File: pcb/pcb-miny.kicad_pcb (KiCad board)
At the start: 2 copper layers, 139.8 x 99.8 mm, 116 parts, among them SW1 Switch, SW10 Switch, SW11 Switch, SW12 Switch, SW13 Switch, SW14 Switch, SW15 Switch, SW16 Switch, SW17 Switch, SW18 Switch, SW19 Switch, SW2 Switch, SW20 Switch, SW21 Switch, SW22 Switch, SW23 Switch, SW24 Switch, SW25 Switch, SW26 Switch, SW27 Switch, SW28 Switch, SW29 Switch, SW3 Switch, SW30 Switch, SW31 Switch, SW32 Switch, SW33 Switch, SW34 Switch, SW4 Switch, SW5 Switch, SW6 Switch, SW7 Switch, SW8 Switch, SW9 Switch

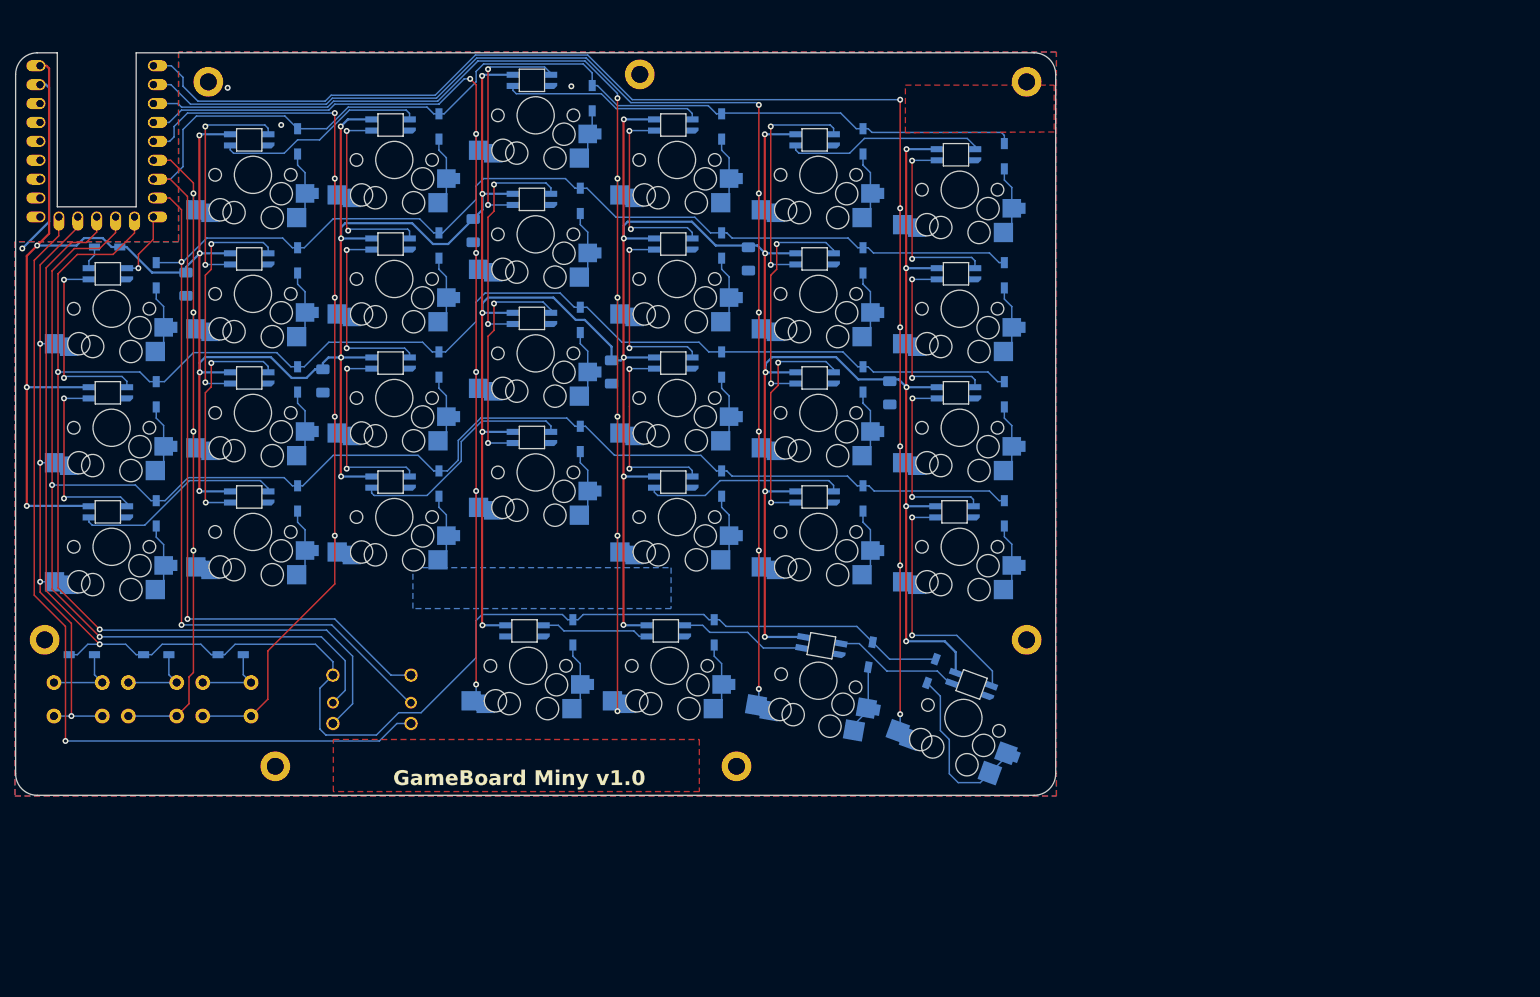
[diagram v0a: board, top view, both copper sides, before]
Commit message: miny-v2 draft
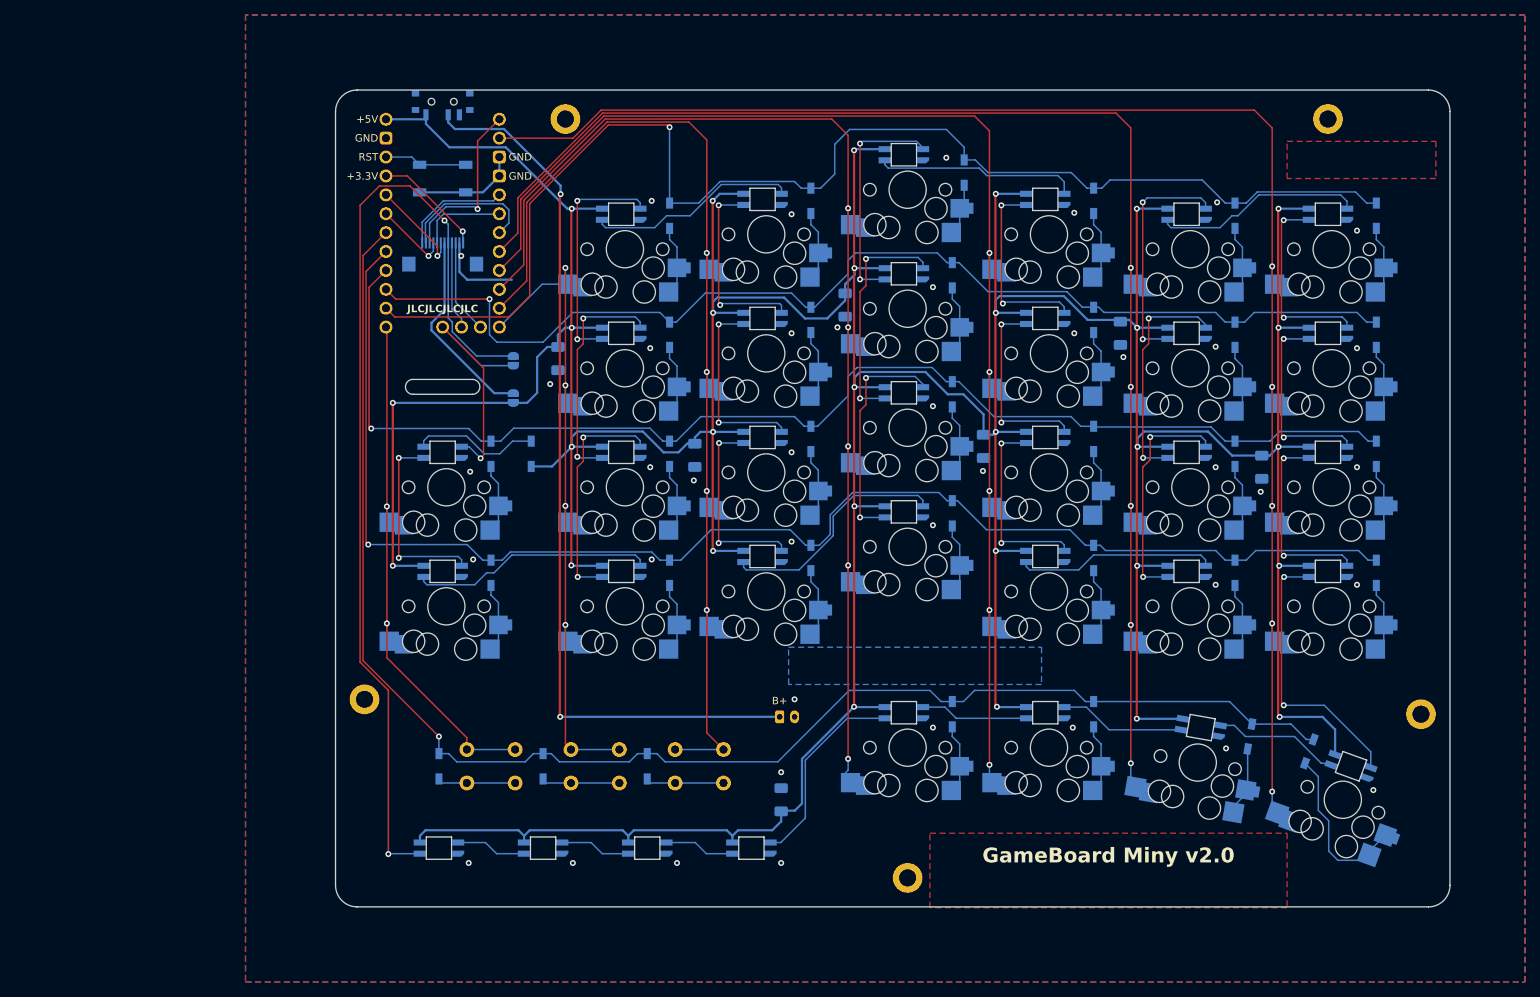
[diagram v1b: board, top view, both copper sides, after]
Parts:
- removed the D7 at (36.5, 100.5)
- removed FiveWay1: 5Way-Tactile_K1-1506DN-01, zzkeeb:Button_5way
- removed the H4 at (101.5, 73.5)
- removed H6: MountingHole, zzkeeb:Hole_M2-TH
- removed the LED1 at (30.0, 100.3)
- removed MCU1: rp2040-zero, zzkeeb:MCU_rp2040-zero-tht
- removed the SW7 at (30.5, 105.0)
- added C7: 100n, Capacitor_SMD:C_1206_3216Metric_Pad1.33x1.80mm_HandSolder, B.Cu at (120.5, 171.0)
- added J1: RP2040, zzkeeb:MCU_rp2040-helios, B.Cu at (75.0, 93.5)
- added J2: Conn_01x02_Socket, zzkeeb:Connector_JST-1x02-2.00mm, F.Cu at (120.3, 159.8)
- added JP2: VIK 5V, Jumper:SolderJumper-2_P1.3mm_Open_RoundedPad1.0x1.5mm, B.Cu at (84.5, 117.0)
- added JP4: VIK LED, Jumper:SolderJumper-2_P1.3mm_Open_RoundedPad1.0x1.5mm, B.Cu at (84.5, 112.0)
- added LED31: YS-SK6812MINI-E, zzkeeb:LED_SK6812-MINI-E, B.Cu at (116.5, 177.5)
- added LED32: YS-SK6812MINI-E, zzkeeb:LED_SK6812-MINI-E, B.Cu at (102.5, 177.5)
- added LED33: YS-SK6812MINI-E, zzkeeb:LED_SK6812-MINI-E, B.Cu at (88.5, 177.5)
- added LED34: YS-SK6812MINI-E, zzkeeb:LED_SK6812-MINI-E, B.Cu at (74.5, 177.5)
- added RST1: SW_Push, zzkeeb:Button_SW_SPST_SKQG_WithoutStem, B.Cu at (75.0, 87.5)
- added SW34: SW_SPDT, zzkeeb:Switch_SPDT-PCM12, B.Cu at (75.0, 77.5)
- added VIK_K1: Connector_VIK-keyboard, zzkeeb:Connector_VIK-horizontal-keyboard, B.Cu at (75.0, 97.7)
- moved SW29 64.1 mm to (109.5, 166.5), turned to 180 degrees
- moved D34 63.4 mm to (86.9, 124.5), turned to -90 degrees
- moved SW28 60.2 mm to (95.5, 166.5), turned to 180 degrees
- moved D29 58.0 mm to (102.5, 166.5), turned to -90 degrees
- moved SW27 56.2 mm to (81.5, 166.5), turned to 180 degrees
- moved D28 54.1 mm to (88.5, 166.5), turned to -90 degrees
- moved H5 53.9 mm to (206.5, 159.5)
- moved D30 52.2 mm to (143.5, 159.5)
- moved D31 52.2 mm to (162.5, 159.5)
- moved D32 52.2 mm to (183.5, 162.5)
- moved LED27 52.2 mm to (197.1, 166.5)
- moved LED28 52.2 mm to (176.9, 161.3)
- moved LED29 52.2 mm to (156.0, 159.3)
- moved LED30 52.2 mm to (137.0, 159.3)
- moved SW30 52.2 mm to (137.5, 164.0)
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- renumbered D11 to D10, D12 to D11, D13 to D12, D14 to D13, D15 to D14, D16 to D15, D17 to D16, D18 to D17, D19 to D18, D20 to D19, D21 to D20, D22 to D21, D23 to D22, D24 to D23, D25 to D24, D26 to D25, D27 to D26, D28 to D27, D29 to D28, D30 to D29, D31 to D30, D32 to D31, D33 to D32, D34 to D33, D40 to D34, D8 to D7, D9 to D8, D10 to D9, H7 to H4, LED2 to LED1, LED11 to LED10, LED12 to LED11, LED13 to LED12, LED14 to LED13, LED15 to LED14, LED16 to LED15, LED17 to LED16, LED18 to LED17, LED19 to LED18, LED20 to LED19, LED3 to LED2, LED21 to LED20, LED22 to LED21, LED23 to LED22, LED24 to LED23, LED25 to LED24, LED26 to LED25, LED27 to LED26, LED28 to LED27, LED29 to LED28, LED30 to LED29, LED4 to LED3, LED31 to LED30, LED5 to LED4, LED6 to LED5, LED7 to LED6, LED8 to LED7, LED9 to LED8, LED10 to LED9, SW11 to SW10, SW12 to SW11, SW13 to SW12, SW14 to SW13, SW15 to SW14, SW16 to SW15, SW17 to SW16, SW18 to SW17, SW19 to SW18, SW20 to SW19, SW21 to SW20, SW22 to SW21, SW23 to SW22, SW24 to SW23, SW25 to SW24, SW26 to SW25, SW27 to SW26, SW28 to SW27, SW29 to SW28, SW30 to SW29, SW31 to SW30, SW32 to SW31, SW33 to SW32, SW34 to SW33, SW8 to SW7, SW9 to SW8, SW10 to SW9
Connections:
- D34 pad 1: Net-(D40-K) -> Net-(D34-K)
- LED1 pad 1: +5V -> Net-(D34-K)
- LED1 pad 4: Net-(LED1-DOUT) (its old number) -> LED
- LED30 pad 2: unconnected-(LED31-DOUT-Pad2) -> Net-(LED30-DOUT)
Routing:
- net LED_OUT: track 0.00 -> 131.8 mm, vias 0 -> 2
- net col7: track 121.0 -> 0.00 mm, vias 1 -> 0
- net BAT: track 0.00 -> 120.6 mm, vias 0 -> 2
- net row2: track 252.2 -> 171.5 mm, vias 2 -> 1
- net +5V: track 714.9 -> 793.7 mm, vias 31 -> 30
- net row1: track 222.5 -> 152.5 mm, vias 2 -> 1
- net row3: track 247.5 -> 189.8 mm, vias 2 -> 1
- net row0: track 228.4 -> 176.3 mm
- net VIK_5V_1: track 0.00 -> 27.0 mm
- net Net-(LED30-DOUT): track 0.00 -> 26.9 mm
- net Net-(LED1-DOUT) (its old number): track 26.2 -> 0.00 mm, vias 2 -> 0
- net LED: track 9.28 -> 34.4 mm
- net SPI_CS: track 0.00 -> 23.4 mm, vias 0 -> 1
- net col3: track 138.6 -> 158.0 mm, vias 6 -> 5
- net SPI_MISO: track 0.00 -> 18.9 mm
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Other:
- board size 139.8 x 99.8 mm -> 149.8 x 109.8 mm
- board text added: "CLK"
- board text added: "CS"
- board text added: "GPIO1"
- board text added: "GPIO2"
- board text added: "GameBoard Miny v2.0"
- board text added: "MISO"
- board text added: "MOSI"
- board text added: "SCL"
- board text added: "SDA"
- board text removed: "C7"
- board text removed: "GameBoard Miny v1.0"
